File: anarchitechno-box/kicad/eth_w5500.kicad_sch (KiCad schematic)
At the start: 35 parts, among them U16 W5500, U17 ARJM11B1-009-AB-EW2, Y1 25MHz

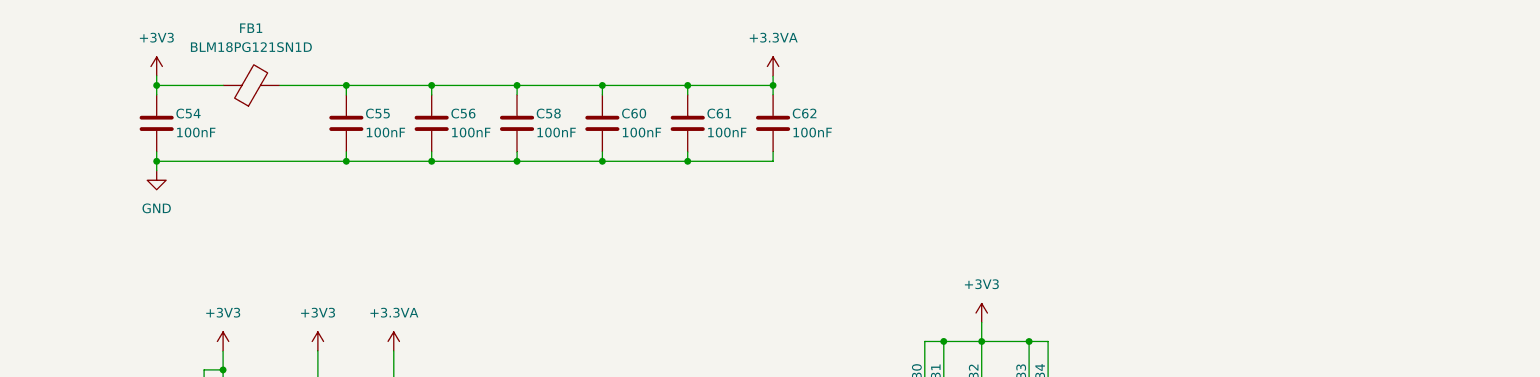
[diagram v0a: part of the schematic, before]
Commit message: trein trein trein
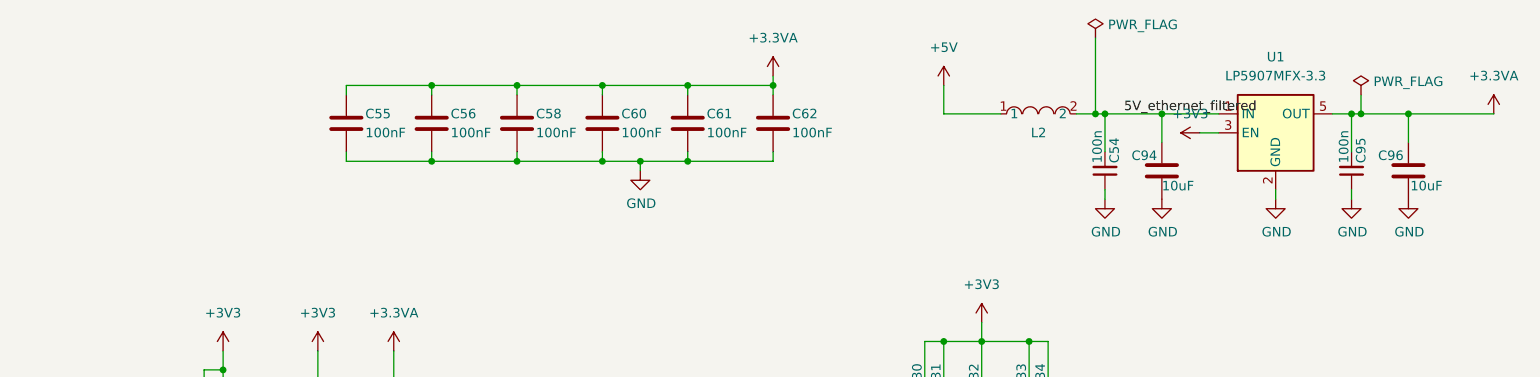
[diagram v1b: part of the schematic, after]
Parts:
- removed C54: 100nF, Capacitor_SMD:C_0402_1005Metric, symbol Device:C
- removed FB1: BLM18PG121SN1D, Inductor_SMD:L_0603_1608Metric, symbol Device:FerriteBead
- added C54, C95: 100n, Capacitor_SMD:C_0402_1005Metric, symbol Device:C_Small
- added C94, C96: 10uF, Capacitor_SMD:C_0603_1608Metric, symbol Device:C
- added L2: BLM18PG121SN1D_C14709, BigFishImports:L0603, symbol BigFishImports:BLM18PG121SN1D_C14709
- added U1: LP5907MFX-3.3, Package_TO_SOT_SMD:SOT-23-5, symbol Regulator_Linear:LP5907MFX-3.3
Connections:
- net +3.3VA: now also C95.2, C96.1, U1.5 (OUT)
- net +3V3: now also U1.3 (EN)
- net GND: now also C54.1, C94.2, C95.1, C96.2, U1.2 (GND)
- new net +5V: L2.1
- new net 5V_ethernet_filtered: C54.2, C94.1, L2.2, U1.1 (IN)
